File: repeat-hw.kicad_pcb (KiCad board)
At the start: 2 copper layers, 4 parts, among them J1 RB1-125BAG1A, U1 nRF5340-QKxx, U2 W5100, Y1 32MHz

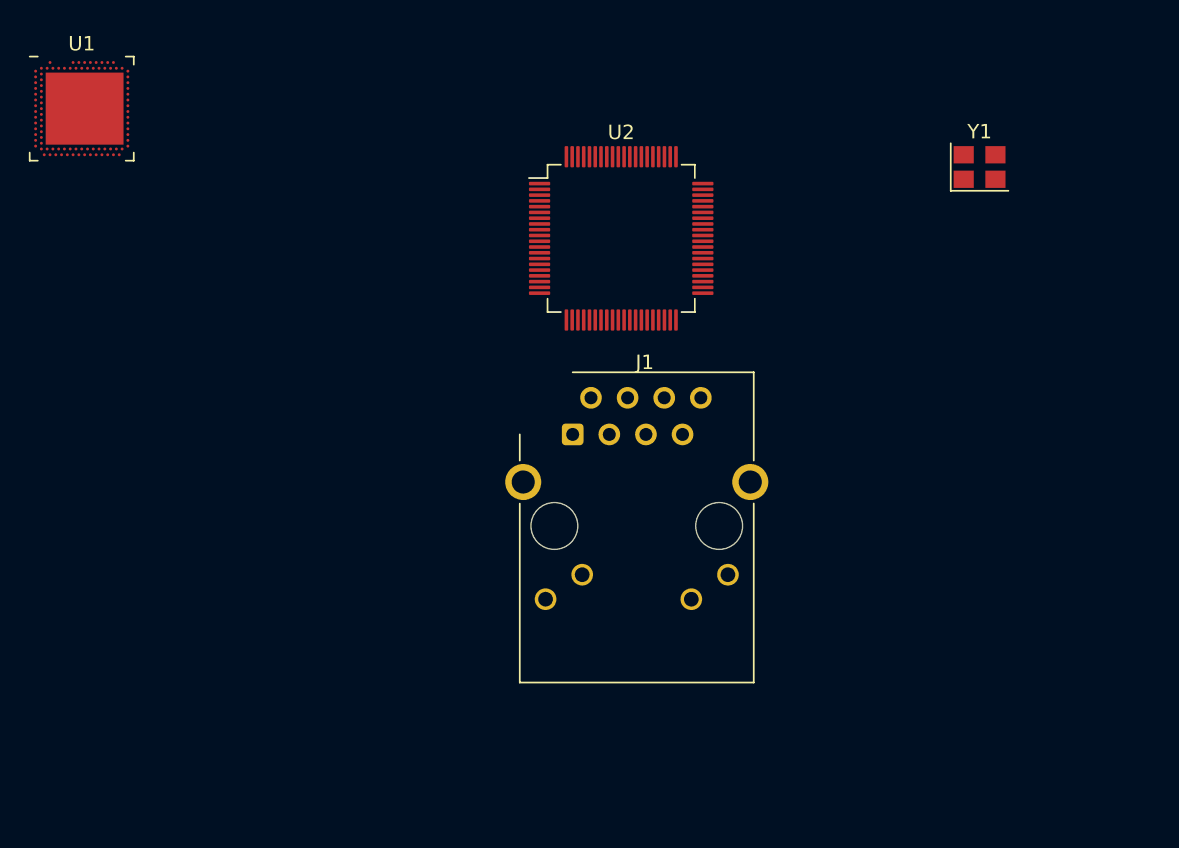
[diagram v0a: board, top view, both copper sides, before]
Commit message: Finishe PoE and ethernet
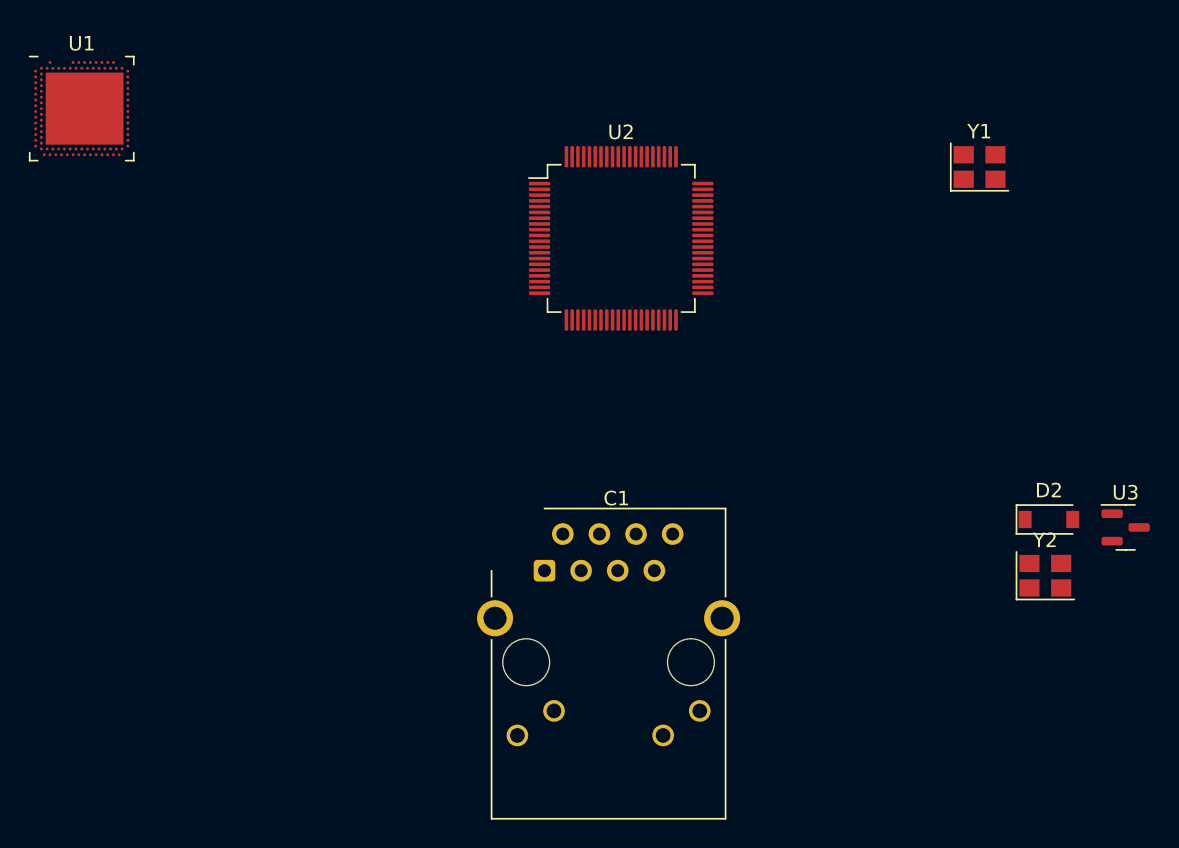
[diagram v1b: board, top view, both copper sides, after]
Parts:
- removed J1: RB1-125BAG1A, Connector_RJ:RJ45_Cetus_J1B1211CCD_Horizontal
- added C1: 4u7, Connector_RJ:RJ45_Cetus_J1B1211CCD_Horizontal, F.Cu at (77.7, 63.0)
- added D2: 1N4148W, Diode_SMD:D_SOD-123, F.Cu at (112.7, 59.5)
- added U3: TLV431DBZ, Package_TO_SOT_SMD:SOT-23, F.Cu at (118.0, 60.0)
- added Y2: 25MHz, Crystal:Crystal_SMD_3225-4Pin_3.2x2.5mm, F.Cu at (112.4, 63.4)
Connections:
- net Net-(U2-Pad10) renamed GNDA
- net Net-(U2-Pad12) renamed +3V3
- net Net-(U2-Pad7) renamed +1V8A
- U2 pad 1: unconnected-(U2-Pad1) -> Net-(U2-Pad1)
- U2 pad 11: unconnected-(U2-Pad11) -> +1V8
- U2 pad 13: Net-(U2-Pad13) -> GND
- U2 pad 14: Net-(U2-Pad13) -> GND
- U2 pad 15: Net-(U2-Pad15) -> +1V8
- U2 pad 16: Net-(U2-Pad15) -> +1V8
- U2 pad 17: Net-(U2-Pad13) -> GND
- U2 pad 2: unconnected-(U2-Pad2) -> +3V3A
- U2 pad 27: unconnected-(U2-Pad27) -> /W5100 + PoE/MISO
- U2 pad 28: unconnected-(U2-Pad28) -> /W5100 + PoE/MOSI
- U2 pad 29: unconnected-(U2-Pad29) -> /W5100 + PoE/~{CS}
- U2 pad 30: unconnected-(U2-Pad30) -> /W5100 + PoE/CLK
- U2 pad 31: unconnected-(U2-Pad31) -> Net-(U2-Pad31)
- U2 pad 32: Net-(U2-Pad13) -> GND
- U2 pad 33: Net-(U2-Pad15) -> +1V8
- U2 pad 34: unconnected-(U2-Pad34) -> GND
- U2 pad 35: unconnected-(U2-Pad35) -> GND
- U2 pad 36: unconnected-(U2-Pad36) -> GND
- U2 pad 37: unconnected-(U2-Pad37) -> GND
- U2 pad 43: Net-(U2-Pad13) -> GND
- U2 pad 5: unconnected-(U2-Pad5) -> /W5100 + PoE/RD+
- U2 pad 56: unconnected-(U2-Pad56) -> /W5100 + PoE/~{INT}
- U2 pad 59: unconnected-(U2-Pad59) -> /W5100 + PoE/~{RST}
- U2 pad 6: unconnected-(U2-Pad6) -> /W5100 + PoE/RD-
- U2 pad 63: unconnected-(U2-Pad63) -> GND
- U2 pad 64: unconnected-(U2-Pad64) -> GND
- U2 pad 65: unconnected-(U2-Pad65) -> GND
- U2 pad 66: unconnected-(U2-Pad66) -> /W5100 + PoE/LINK
- U2 pad 68: Net-(U2-Pad13) -> GND
- U2 pad 69: Net-(U2-Pad15) -> +1V8
- U2 pad 70: unconnected-(U2-Pad70) -> /W5100 + PoE/FDX
- U2 pad 75: unconnected-(U2-Pad75) -> Net-(U2-Pad75)
- U2 pad 76: unconnected-(U2-Pad76) -> Net-(U2-Pad76)
- U2 pad 8: unconnected-(U2-Pad8) -> /W5100 + PoE/TD+
- U2 pad 9: unconnected-(U2-Pad9) -> /W5100 + PoE/TD-
